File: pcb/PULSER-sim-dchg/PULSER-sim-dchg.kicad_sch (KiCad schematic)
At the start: 17 parts, among them Q1 IRF640, U1 ${SIM.PARAMS}, U2 ${SIM.PARAMS}

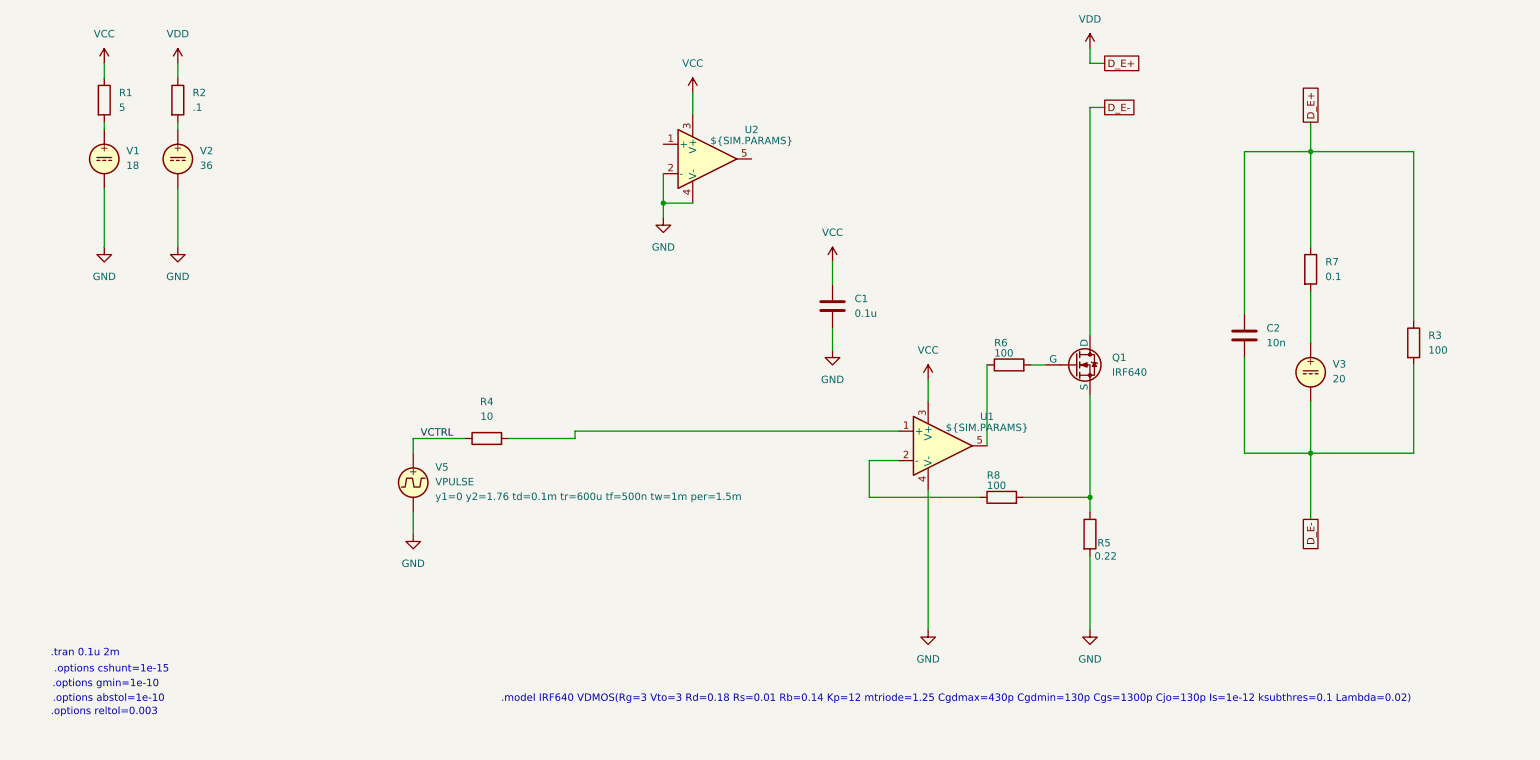
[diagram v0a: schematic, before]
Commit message: PULSER r2 pulse shaper draft
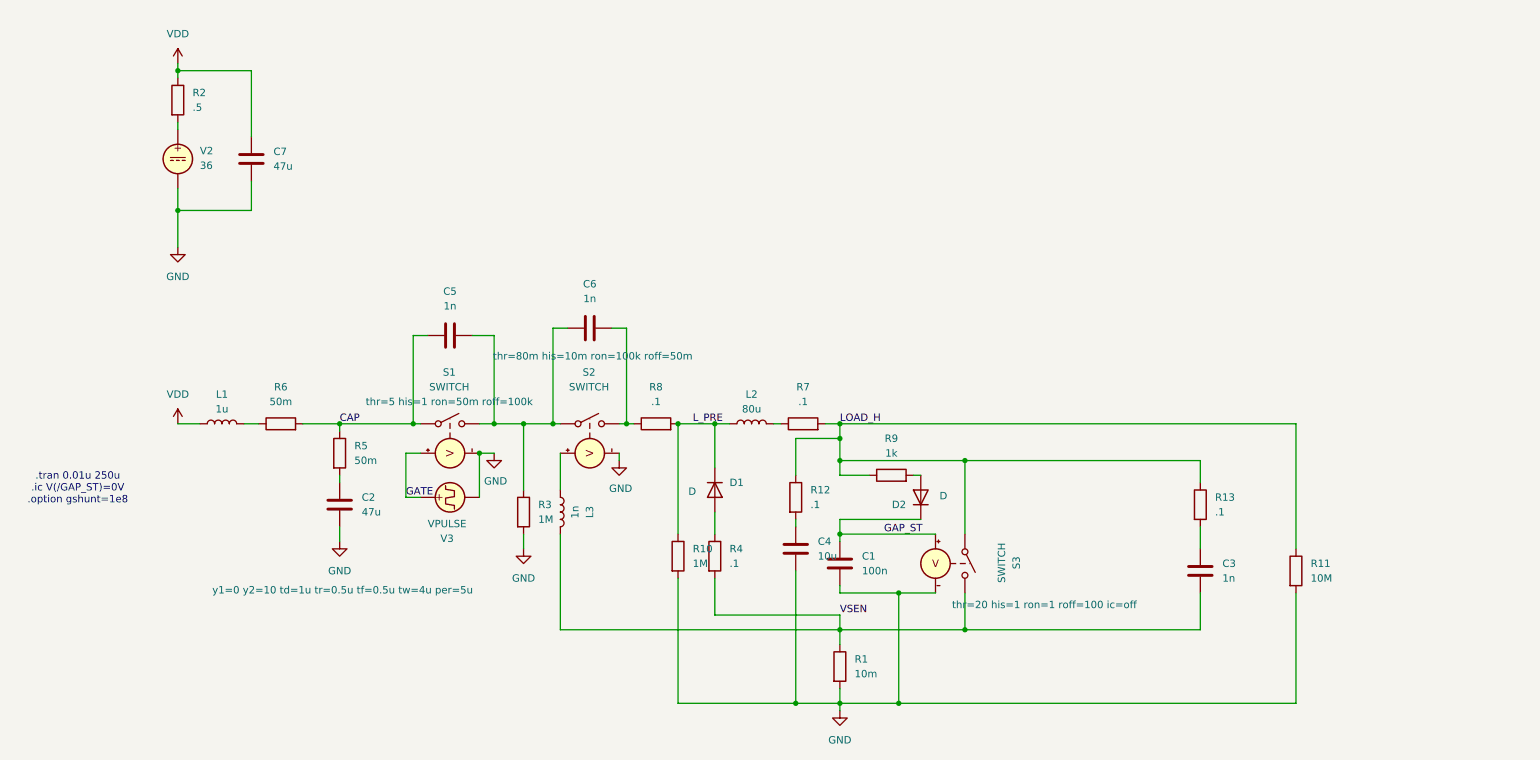
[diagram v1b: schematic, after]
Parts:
- removed Q1: IRF640, symbol Simulation_SPICE:NMOS
- removed U1, U2: ${SIM.PARAMS}, symbol Simulation_SPICE:OPAMP
- removed V1: 18, symbol Simulation_SPICE:VDC
- removed V3: 20, symbol Simulation_SPICE:VDC
- removed V5: VPULSE, symbol Simulation_SPICE:VPULSE
- added C3, C5, C6: 1n, symbol Device:C
- added C4: 10u, symbol Device:C
- added C7: 47u, symbol Device:C
- added D1, D2: D, symbol Device:D
- added L1: 1u, symbol Device:L
- added L2: 80u, symbol Device:L
- added L3: 1n, symbol Device:L
- added R10: 1M, symbol Device:R
- added R11: 10M, symbol Device:R
- added R12, R13: .1, symbol Device:R
- added R9: 1k, symbol Device:R
- added S1, S2, S3: SWITCH, symbol Simulation_SPICE:SWITCH
- added V3: VPULSE, symbol Simulation_SPICE:VPULSE
- C1: value 0.1u -> 100n; footprint Capacitor_SMD:C_0603_1608Metric -> (none)
- C2: value 10n -> 47u
- R1: value 5 -> 10m
- R2: value .1 -> .5
- R3: value 100 -> 1M
- R4: value 10 -> .1
- R5: value 0.22 -> 50m; footprint Resistor_SMD:R_0603_1608Metric -> (none)
- R6: value 100 -> 50m; footprint Resistor_SMD:R_0603_1608Metric -> (none)
- R7: value 0.1 -> .1
- R8: value 100 -> .1; footprint Resistor_SMD:R_0603_1608Metric -> (none)
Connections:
- net GND: now also C1.1, C2.1, R1.2, R3.2, C4.1, C7.1, R10.2, R11.2, S1.4 (C-), S2.4 (C-), S3.4 (C-), V3.2; no longer C1.2, R5.2
- net VDD: now also C7.2, L1.1; no longer C2.1, R3.1, R7.1
- net VSEN: now reaches R4.2
- net VSEN: now also R1.1, C3.1, L3.2, S3.2 (N-)
- net at R8.1: now also C6.1, S2.2 (N-)
- net at R6.1: now also L1.2
- net LOAD_H: now reaches R7.2
- net LOAD_H: now also R11.1, R12.1, R13.1, R9.1, S3.1 (N+)
- net CAP: now reaches R6.2
- net CAP: now also R5.1, C5.2, S1.1 (N+)
- net L_PRE: now reaches R8.2
- net L_PRE: now also D1.1 (K), L2.1, R10.1; no longer R5.1
- net D_E-: no longer names the net of C2.2
- net D_E-: now also R5.2; no longer R3.2
- removed net VCC: C1.1, R1.1
- net VCTRL: no longer names the net of R4.1
- net VCTRL: now also D1.2 (A)
- new net: C5.1, C6.2, R3.1, S1.2 (N-), S2.1 (N+)
- new net: L3.1, S2.3 (C+)
- new net: D2.2 (A), R9.2
- new net: C3.2, R13.2
- new net: C4.2, R12.2
- new net: L2.2, R7.1
- new net GAP_ST: C1.2, D2.1 (K), S3.3 (C+)
- new net GATE: S1.3 (C+), V3.1
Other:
- note added: ".tran 0.01u 250u .ic V(/GAP_ST)=0V .option gshunt=1e8"
- note removed: ".model IRF640 VDMOS(Rg=3 Vto=3 Rd=0.18 Rs=0.01 Rb=0.14 Kp=12 mtriode=1.25 Cgdmax=430p Cgdmin=130p Cgs=1300p Cjo=130p Is=1e-12 ksubthres=0.1 Lambda=0.02)"
- note removed: ".options abstol=1e-10"
- note removed: ".options cshunt=1e-15"
- note removed: ".options gmin=1e-10"
- note removed: ".options reltol=0.003"
- note removed: ".tran 0.1u 2m"
